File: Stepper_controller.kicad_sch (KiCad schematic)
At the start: 29 parts, among them J6 Encoder connector, J7 Motor connector, U3 TMC5130A-TA

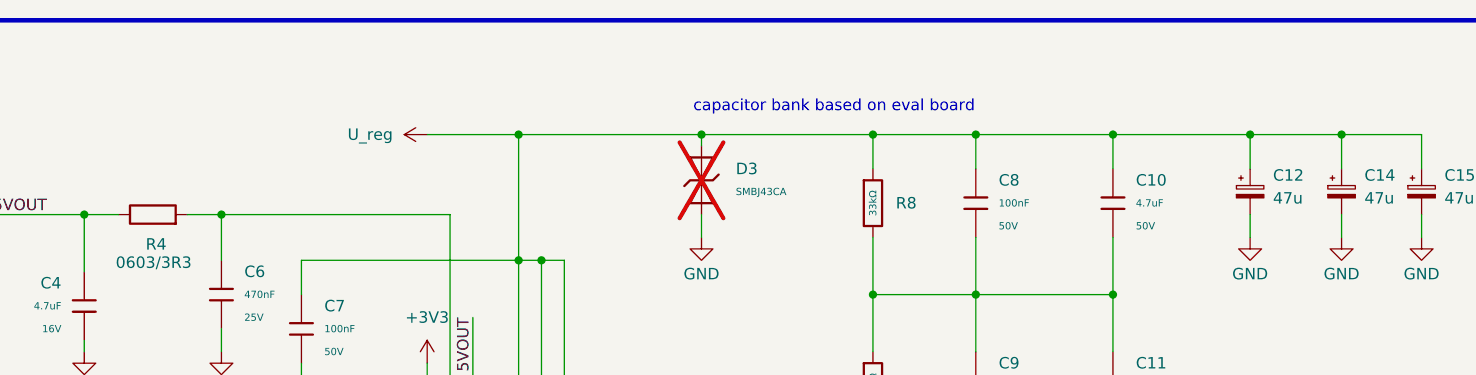
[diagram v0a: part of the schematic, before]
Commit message: updated routing
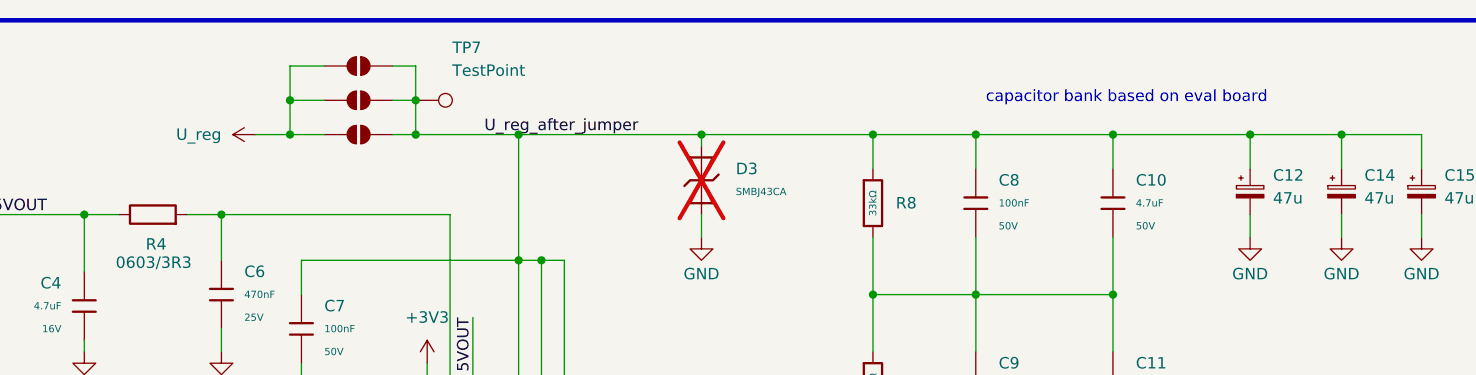
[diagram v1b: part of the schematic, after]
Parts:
- added JP1, JP2, JP3: SolderJumper_2_Open, Jumper:SolderJumper-2_P1.3mm_Open_TrianglePad1.0x1.5mm, symbol Jumper:SolderJumper_2_Open
- added TP7: TestPoint, TestPoint:TestPoint_Pad_D1.0mm, symbol Connector:TestPoint
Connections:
- net U_reg: now also JP1.1 (A), JP2.1 (A), JP3.1 (A); no longer C10.1, C12.1, C14.1, C15.1, C7.1, C8.1, D3.2, R8.1, U3.21 (VS), U3.39 (VSA), U3.40 (VS)
- new net U_reg_after_jumper: C10.1, C12.1, C14.1, C15.1, C7.1, C8.1, D3.2, JP1.2 (B), JP2.2 (B), JP3.2 (B), R8.1, TP7.1, U3.21 (VS), U3.39 (VSA), U3.40 (VS)
